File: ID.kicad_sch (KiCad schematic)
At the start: 25 parts

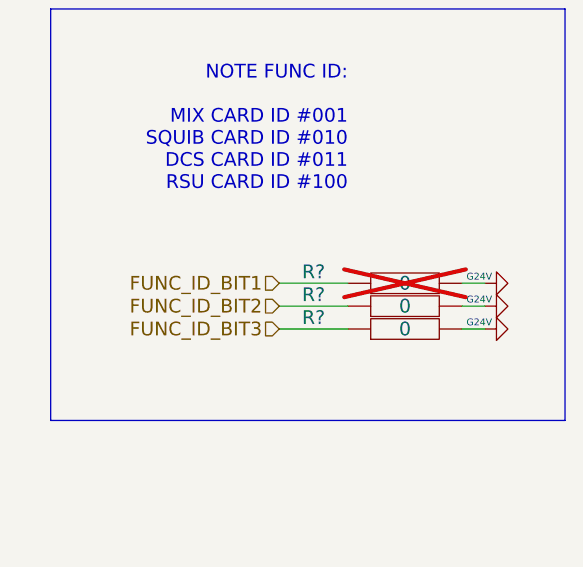
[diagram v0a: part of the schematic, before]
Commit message: assembly
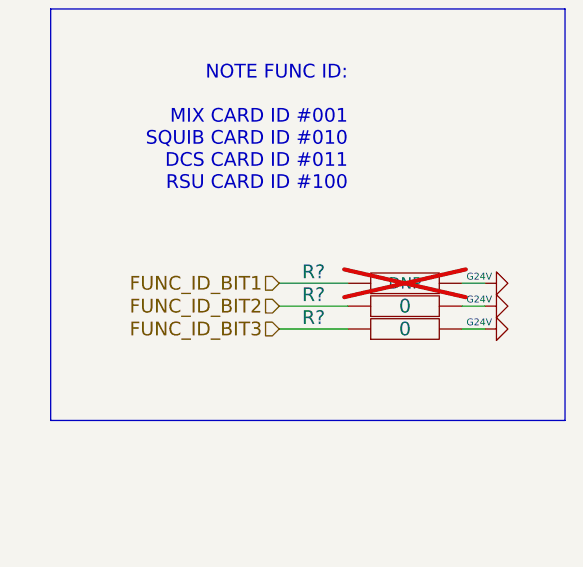
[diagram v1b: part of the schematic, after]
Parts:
- R?: fit_field (none) -> DNP
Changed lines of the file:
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@@
-(kicad_sch (version 20230121) (generator eeschema)
+(kicad_sch (version 20230409) (generator eeschema)
   (paper "A3")
   (title_block
